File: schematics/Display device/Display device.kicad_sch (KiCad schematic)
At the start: 13 parts, among them M2 Stepper_Motor_unipolar_5pin, SW1 SW_DPST, SW2 Button, U1 XIAO ESP32-C3, U2 Voltage Regulator, U4 ULN2003

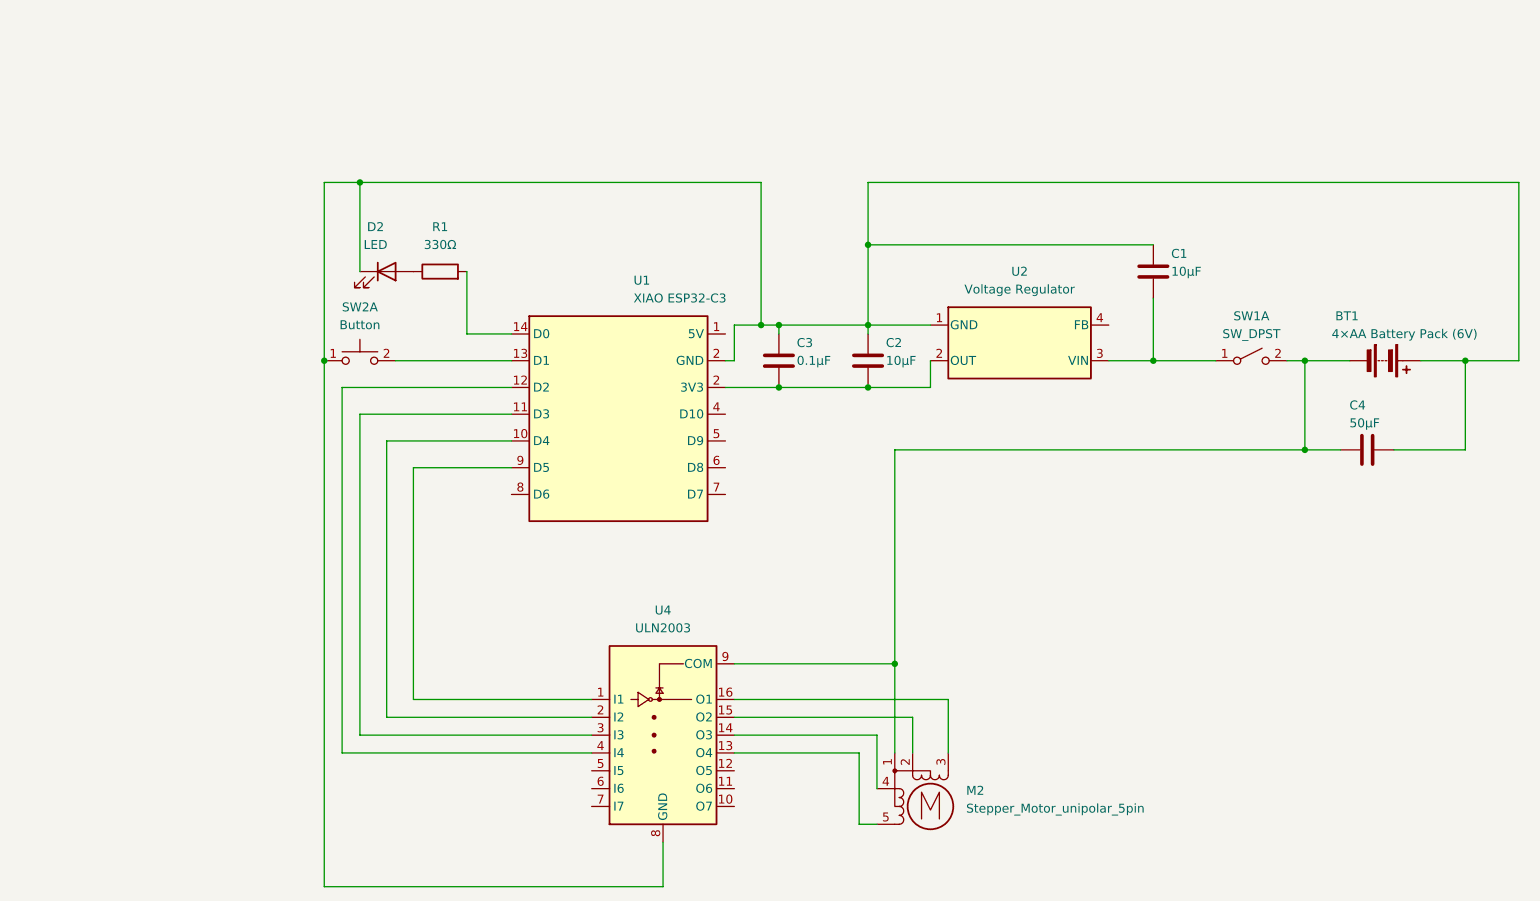
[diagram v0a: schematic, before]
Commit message: update code
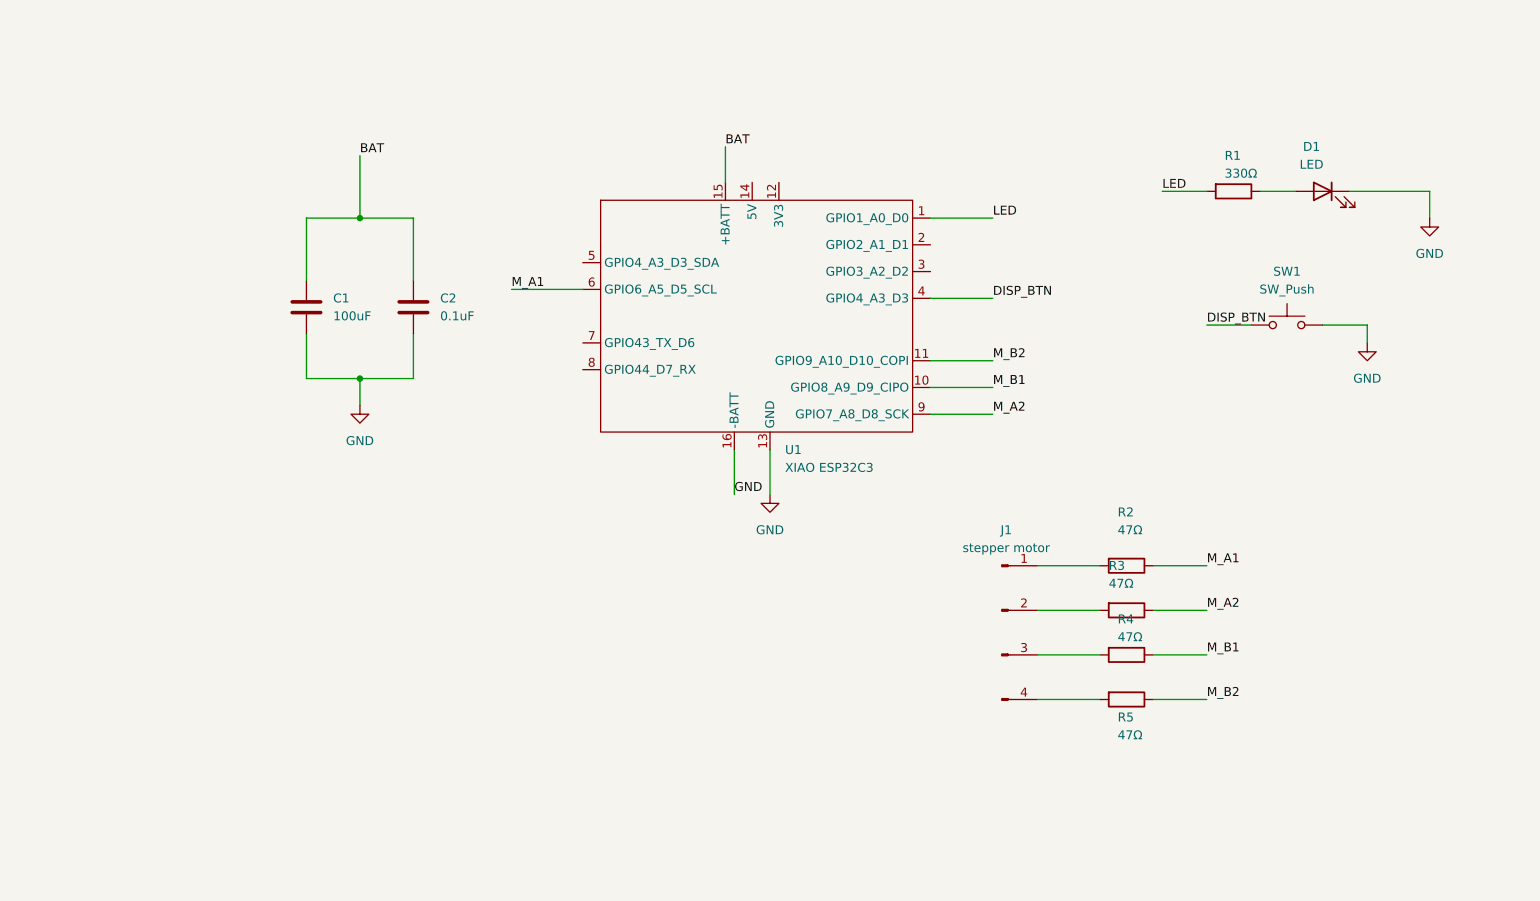
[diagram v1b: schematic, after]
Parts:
- removed BT1: 4×AA Battery Pack (6V), symbol Device:Battery
- removed C3: 0.1µF, symbol Device:C
- removed C4: 50µF, symbol Device:C
- removed D2: LED, symbol Device:LED
- removed M2: Stepper_Motor_unipolar_5pin, symbol Motor:Stepper_Motor_unipolar_5pin
- removed SW1: SW_DPST, symbol Switch:SW_DPST_x2
- removed SW2: Button, symbol Switch:SW_Push_Dual_x2
- removed U1: XIAO ESP32-C3, RF_Module:ESP32-C3-DevKitM-1, symbol RF_Module:ESP32-C3-DevKitM-1
- removed U2: Voltage Regulator, Package_TO_SOT_SMD:TO-263-5_TabPin3, symbol Regulator_Switching:LM2576HVS-3.3
- removed U4: ULN2003, symbol Transistor_Array:ULN2003
- added D1: LED, LED_SMD:LED_0805_2012Metric_Pad1.15x1.40mm_HandSolder, symbol Device:LED
- added J1: stepper motor, Connector_PinHeader_2.54mm:PinHeader_1x04_P2.54mm_Vertical, symbol Connector:Conn_01x04_Pin
- added R2, R3, R4, R5: 47Ω, Resistor_SMD:R_0805_2012Metric_Pad1.20x1.40mm_HandSolder, symbol Device:R
- added SW1: SW_Push, Button_Switch_SMD:SW_Push_1P1T_NO_E-Switch_TL3301NxxxxxG, symbol Switch:SW_Push
- added U1: XIAO ESP32C3, GIX_ESP32:XIAO_ESP32, symbol GIX_ESP32:XIAO_ESP32
- C1: value 10µF -> 100uF; footprint (none) -> Capacitor_SMD:C_0805_2012Metric_Pad1.18x1.45mm_HandSolder
- C2: value 10µF -> 0.1uF; footprint (none) -> Capacitor_SMD:C_0805_2012Metric_Pad1.18x1.45mm_HandSolder
- R1: footprint (none) -> Resistor_SMD:R_0805_2012Metric_Pad1.20x1.40mm_HandSolder
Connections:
- net BAT: now reaches C2.1
- net BAT: now also C1.1, U1.15 (+BATT)
- net GND: now reaches C1.2, C2.2
- net GND: now also D1.1 (K), SW1.2, U1.13 (GND), U1.16 (-BATT)
- net at R1.1: now also D1.2 (A)
- net LED: now reaches R1.2
- net LED: now also U1.1 (GPIO1_A0_D0)
- new net: J1.1 (Pin_1), R2.2
- new net: J1.2 (Pin_2), R3.2
- new net: J1.3 (Pin_3), R4.2
- new net: J1.4 (Pin_4), R5.2
- new net DISP_BTN: SW1.1, U1.4 (GPIO4_A3_D3)
- new net M_A1: R2.1, U1.6 (GPIO6_A5_D5_SCL)
- new net M_A2: R3.1, U1.9 (GPIO7_A8_D8_SCK)
- new net M_B1: R4.1, U1.10 (GPIO8_A9_D9_CIPO)
- new net M_B2: R5.1, U1.11 (GPIO9_A10_D10_COPI)
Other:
- title: Display Device -> Polly Yao_EmoTrace_Display Device

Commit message: kicad update
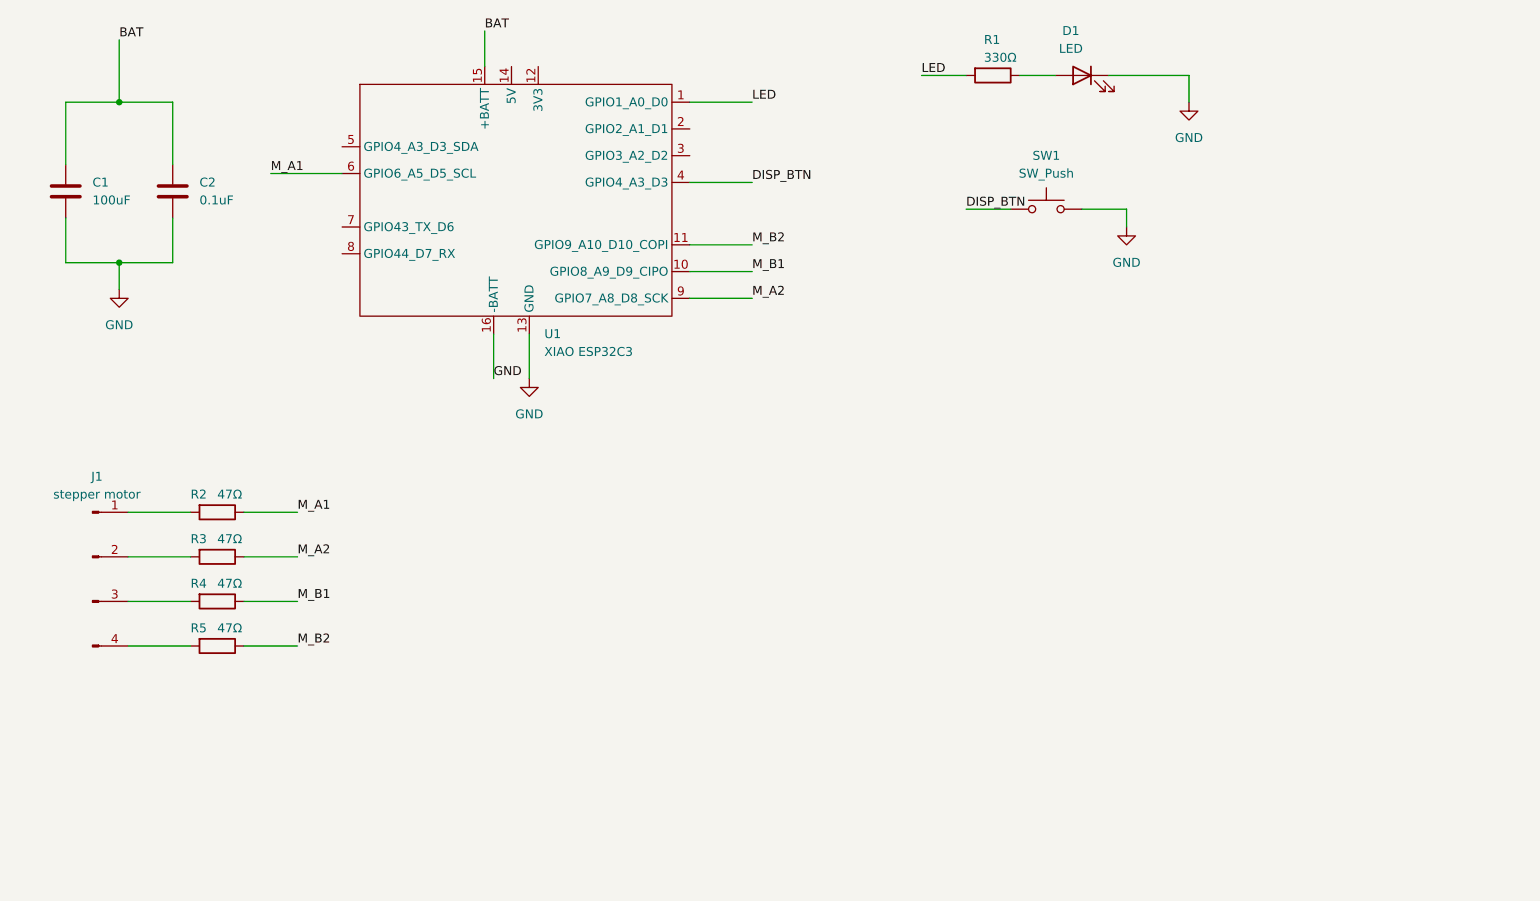
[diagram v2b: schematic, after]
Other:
- moved on the sheet: C1, C2, D1, J1, R1, R2, R3, R4, R5, SW1, U1

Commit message: sche update
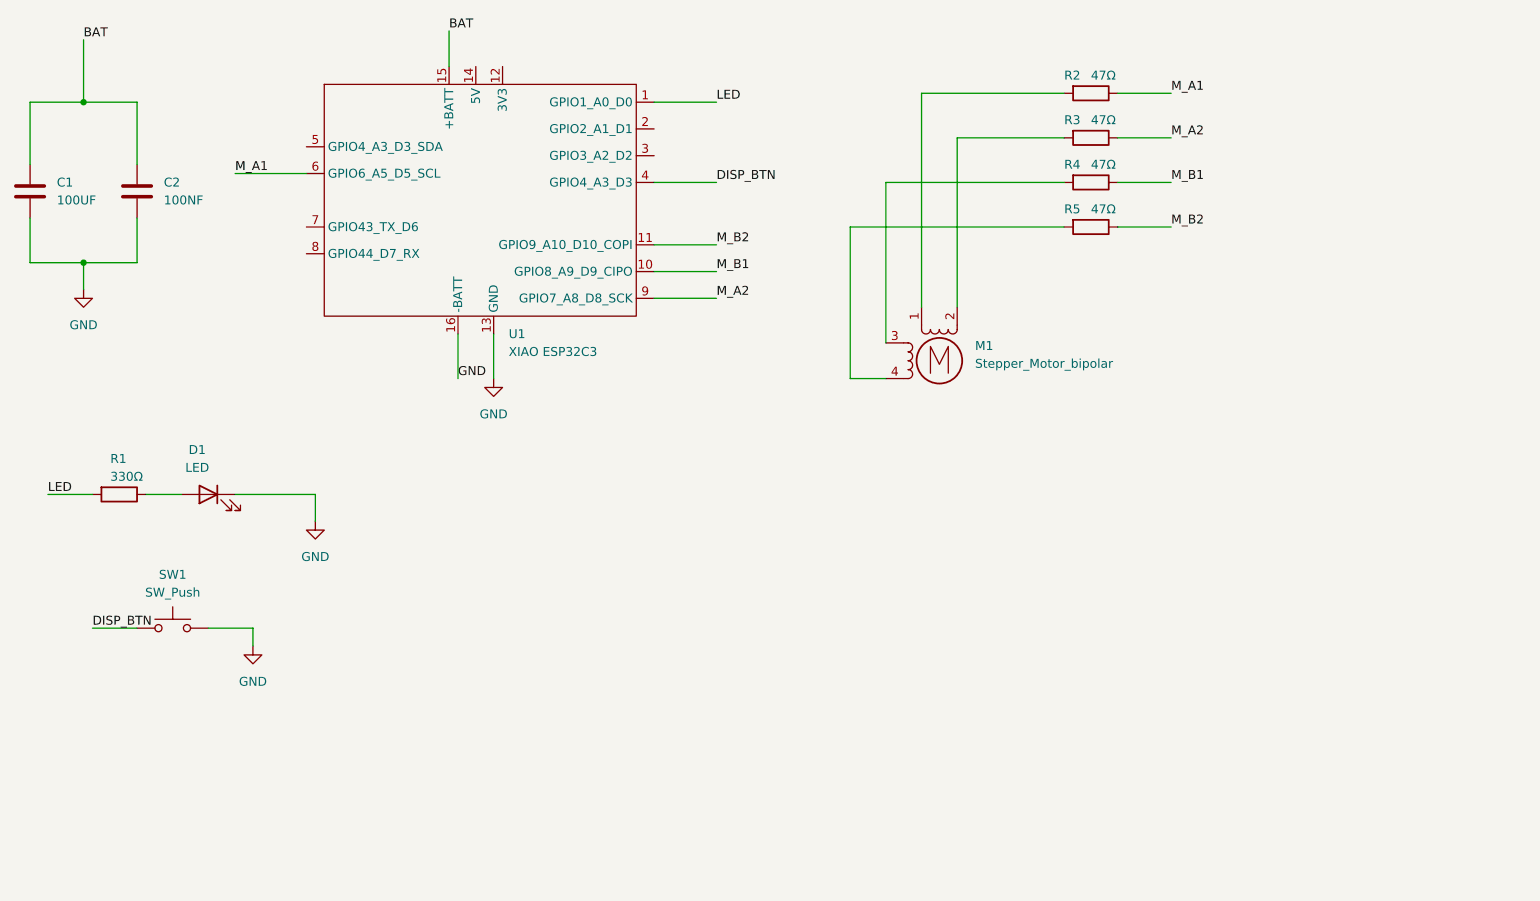
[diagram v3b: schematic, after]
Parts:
- removed J1: stepper motor, Connector_PinHeader_2.54mm:PinHeader_1x04_P2.54mm_Vertical, symbol Connector:Conn_01x04_Pin
- added M1: Stepper_Motor_bipolar, x27_Footprint:x27_stepper_two_holes, symbol Motor:Stepper_Motor_bipolar
- C1: value 100uF -> 100UF
- C2: value 0.1uF -> 100NF
- SW1: footprint Button_Switch_SMD:SW_Push_1P1T_NO_E-Switch_TL3301NxxxxxG -> Button_Switch_SMD:SW_SPST_EVQP7A
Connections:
- net at R2.2: now also M1.1
- net at R3.2: now also M1.2 (-)
- net at R4.2: now also M1.3
- net at R5.2: now also M1.4
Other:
- moved on the sheet: C1, C2, D1, R1, R2, R3, R4, R5, SW1, U1
